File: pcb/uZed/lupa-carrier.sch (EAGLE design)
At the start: 43 parts, among them K1 694108105102

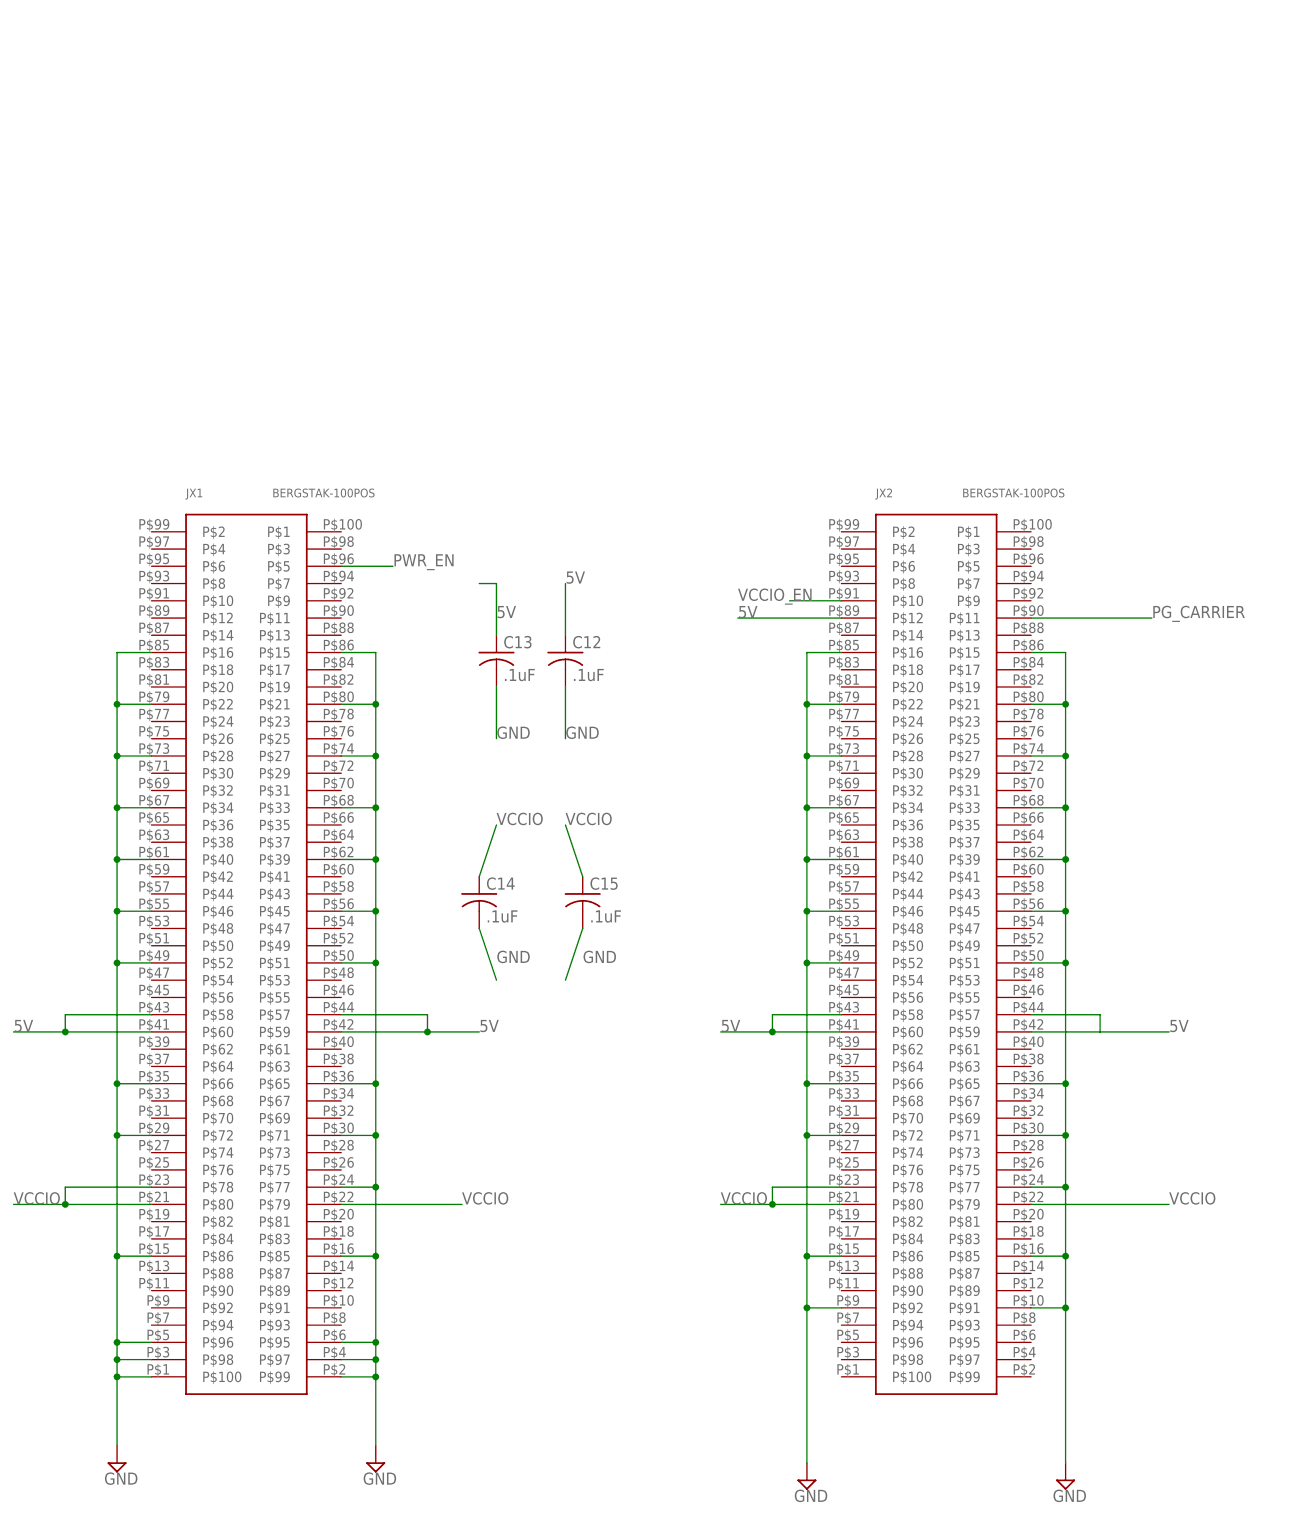
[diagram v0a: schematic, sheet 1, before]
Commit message: more lupa crrier layout work
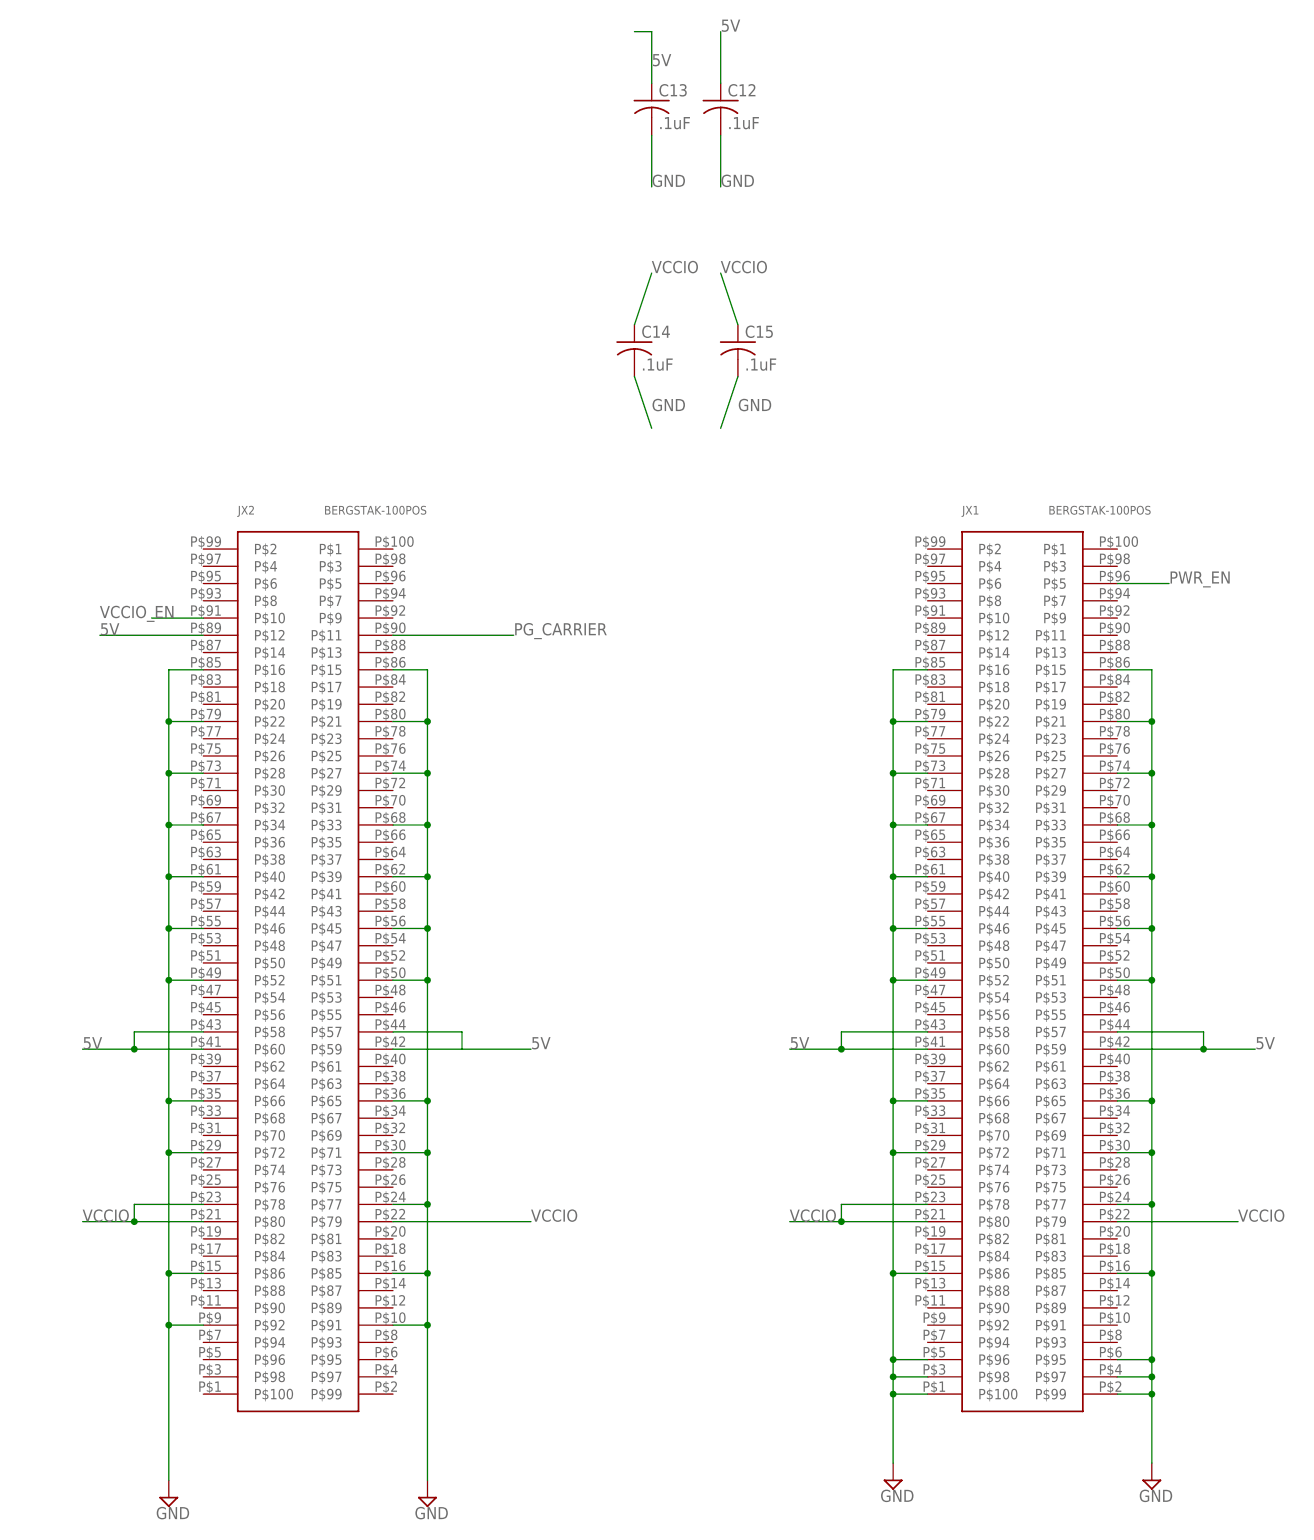
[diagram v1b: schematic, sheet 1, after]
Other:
- moved on the sheet: C12, C13, C14, C15, JX1, JX2
